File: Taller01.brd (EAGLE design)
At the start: 91.3 x 107.2 mm, 19 parts, among them U1 ARDUINO-UNO-R3-SHIELD

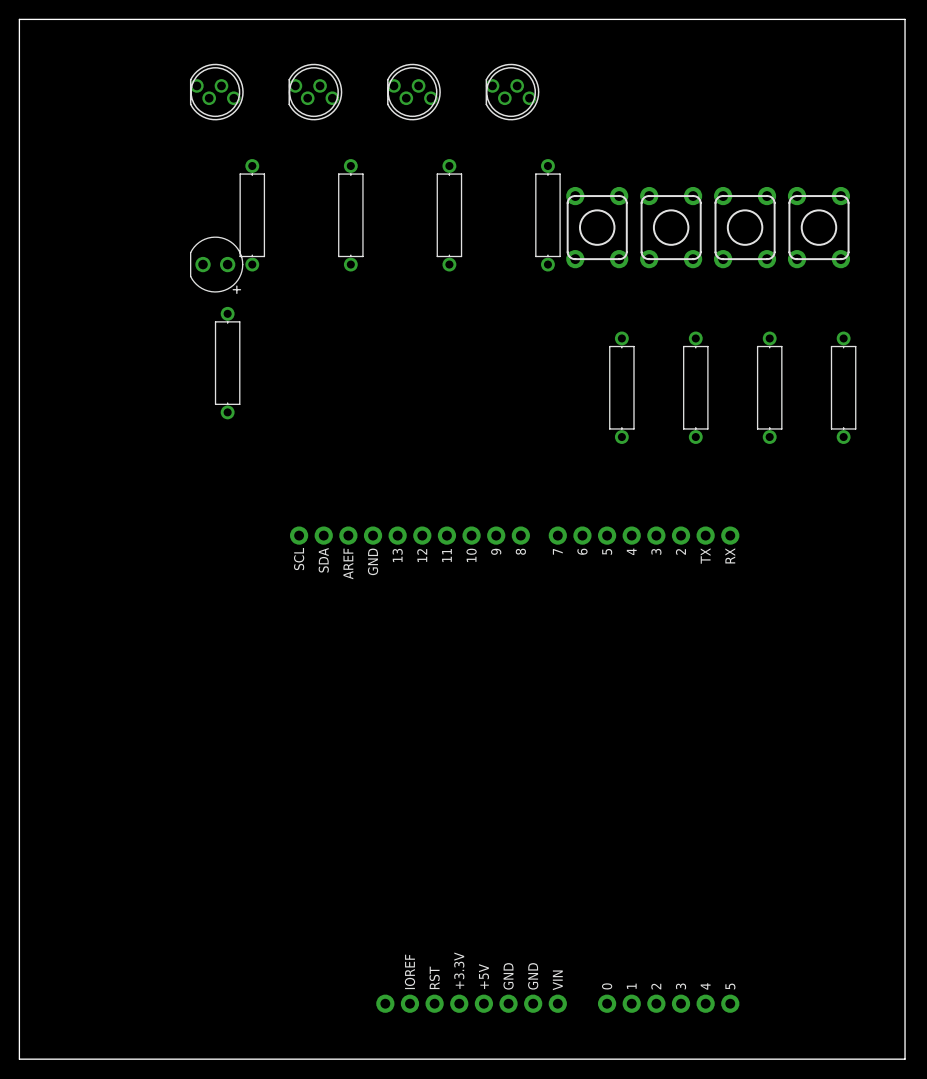
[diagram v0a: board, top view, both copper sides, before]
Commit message: Segundo avance
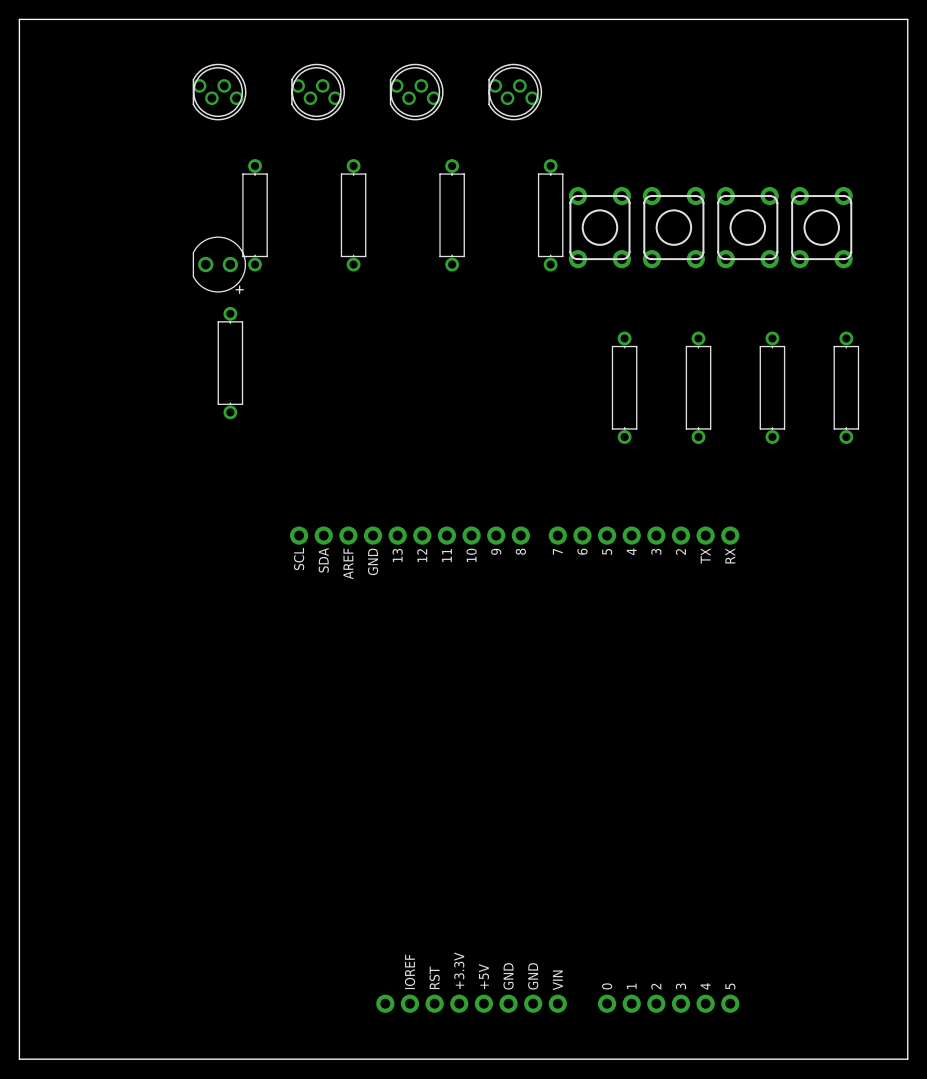
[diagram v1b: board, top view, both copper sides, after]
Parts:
- moved D1 0.28 mm to (20.5, 81.9)
- moved D2 0.28 mm to (51.0, 99.7)
- moved D4 0.28 mm to (30.6, 99.7)
- moved D5 0.28 mm to (20.5, 99.7)
- moved R1 0.28 mm to (62.4, 69.2)
- moved R2 0.28 mm to (21.8, 71.8)
- moved R3 0.28 mm to (70.0, 69.2)
- moved R4 0.28 mm to (77.6, 69.2)
- moved R5 0.28 mm to (85.3, 69.2)
- moved R6 0.28 mm to (54.8, 87.0)
- moved R7 0.28 mm to (44.6, 87.0)
- moved R8 0.28 mm to (34.5, 87.0)
- moved S1 0.28 mm to (59.9, 85.7)
- moved S2 0.28 mm to (67.5, 85.7)
- moved S3 0.28 mm to (75.1, 85.7)
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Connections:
- net U1_GND renamed U1_D13
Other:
- board size 91.3 x 107.2 mm -> 91.6 x 107.2 mm

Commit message: Tercer Avance
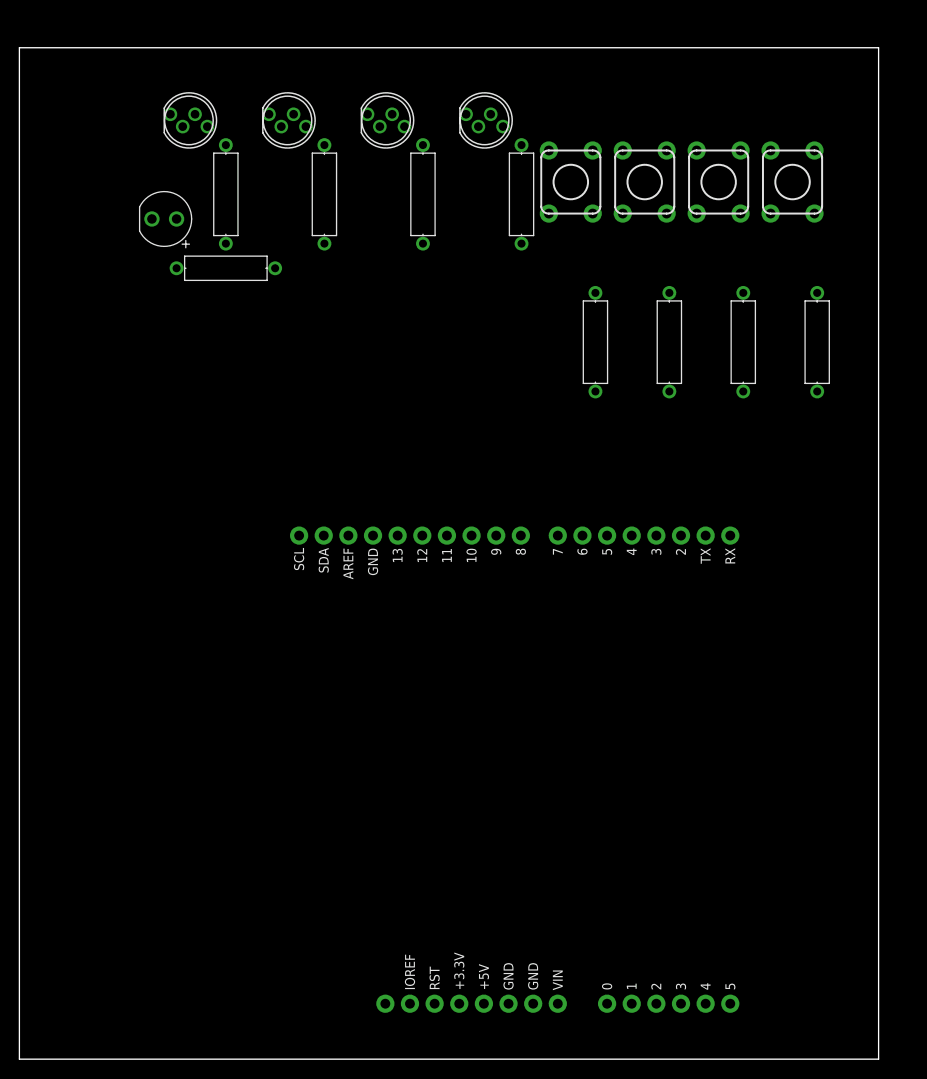
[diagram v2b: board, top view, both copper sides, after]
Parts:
- moved R2 9.79 mm to (21.3, 81.5), turned to 360 degrees
- moved D1 7.27 mm to (14.9, 86.6)
- moved R4 5.58 mm to (74.6, 73.9)
- moved R5 5.58 mm to (82.2, 73.9)
- moved S2 5.58 mm to (64.5, 90.4)
- moved S4 5.58 mm to (79.7, 90.4)
- moved R1 5.58 mm to (59.4, 73.9)
- moved S1 5.58 mm to (56.8, 90.4)
- moved R3 5.58 mm to (67.0, 73.9)
- moved S3 5.58 mm to (72.1, 90.4)
- moved D2 4.19 mm to (48.0, 96.8)
- moved D3 4.19 mm to (37.8, 96.8)
- moved D4 4.19 mm to (27.6, 96.8)
- moved D5 4.19 mm to (17.5, 96.8)
- moved R6 3.70 mm to (51.8, 89.2)
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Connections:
- new net U1_GND: D1.2, D2.C, D3.C, D4.C, D5.C, R1.1, R3.1, R4.1, R5.1, U1.GND@0, U1.GND@1, U1.GND@2
- net D1_A: now also R2.1; no longer R2.2
- net U1_D13: now also R2.2; no longer D1.2, D2.C, D3.C, D4.C, D5.C, R1.1, R3.1, R4.1, R5.1, U1.GND@0, U1.GND@1, U1.GND@2
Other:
- board size 91.6 x 107.2 mm -> 88.6 x 104.3 mm
